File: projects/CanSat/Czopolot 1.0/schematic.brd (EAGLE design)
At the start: 35.6 x 50.8 mm, 12 parts

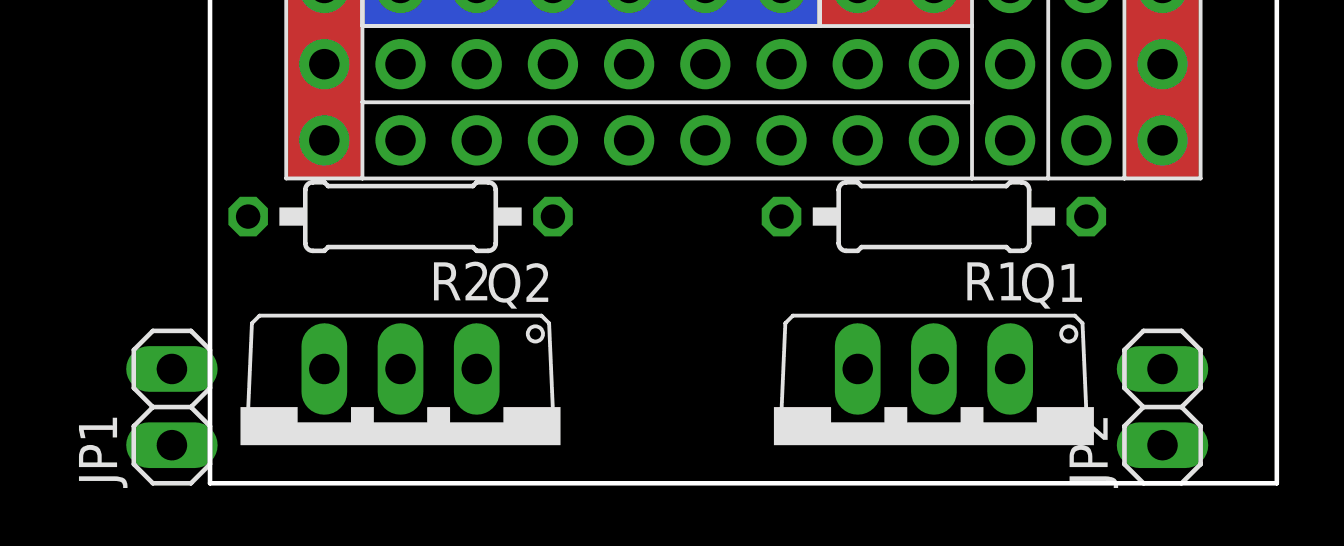
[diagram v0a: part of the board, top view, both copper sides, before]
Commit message: Work work..
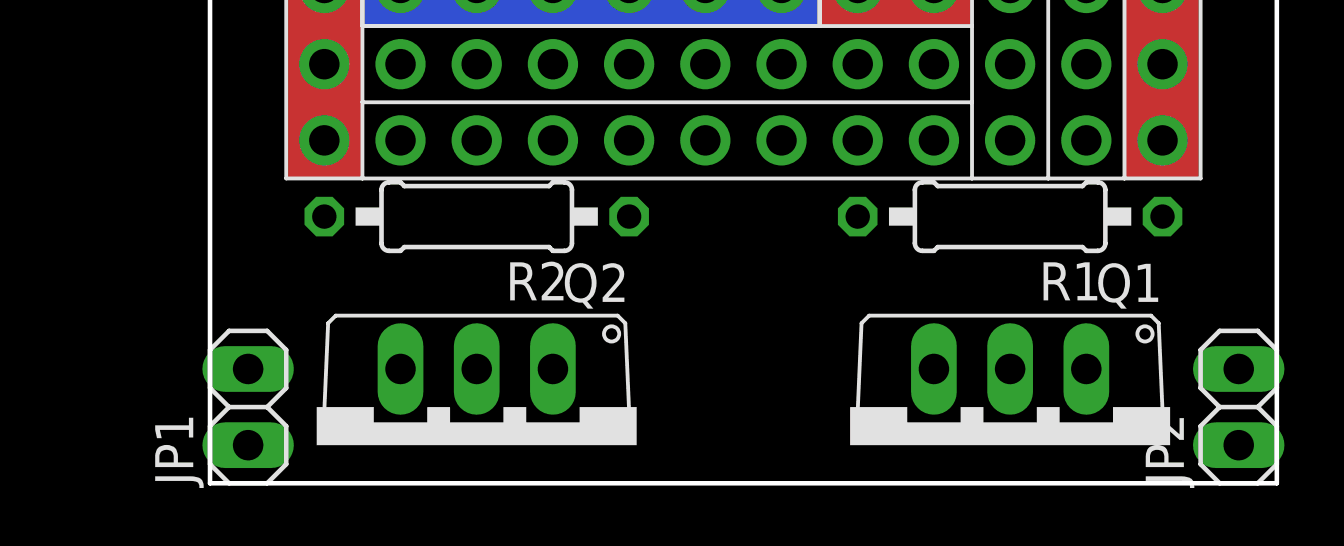
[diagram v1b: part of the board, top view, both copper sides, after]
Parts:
- moved JP1 2.54 mm to (3.81, -48.3)
- moved JP2 2.54 mm to (36.8, -48.3)
- moved Q1 2.54 mm to (29.2, -49.5)
- moved Q2 2.54 mm to (11.4, -49.5)
- moved R1 2.54 mm to (29.2, -41.9)
- moved R2 2.54 mm to (11.4, -41.9)
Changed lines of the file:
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@@
 <?xml version="1.0" encoding="utf-8"?>
 <!DOCTYPE eagle SYSTEM "eagle.dtd">
-<eagle version="9.5.2">
+<eagle version="9.5.1">
 <drawing>
 <settings>
@@
 <element name="U$3" library="SobieskiSat2" package="MODULE_MPU9250" value="MPU9250" x="20.32" y="-8.001" smashed="yes" rot="R270"/>
 <element name="U$4" library="SobieskiSat2" package="MODULE_BMP280" value="BMP280" x="15.24" y="-28.829" smashed="yes" rot="R90"/>
-<element name="R1" library="rcl" library_urn="urn:adsk.eagle:library:334" package="0207/10" package3d_urn="urn:adsk.eagle:package:23491/2" value="" x="26.67" y="-41.91" smashed="yes" rot="R180">
-<attribute name="NAME" x="29.718" y="-43.434" size="1.27" layer="25" ratio="10" rot="R180"/>
-<attribute name="POPULARITY" value="81" x="26.67" y="-41.91" size="1.778" layer="27" rot="R180" display="off"/>
-<attribute name="SPICEPREFIX" value="R" x="26.67" y="-41.91" size="1.778" layer="27" rot="R180" display="off"/>
-<attribute name="VALUE" x="28.9306" y="-41.275" size="1.27" layer="27" ratio="10" rot="R180"/>
-</element>
-<element name="R2" library="rcl" library_urn="urn:adsk.eagle:library:334" package="0207/10" package3d_urn="urn:adsk.eagle:package:23491/2" value="" x="8.89" y="-41.91" smashed="yes" rot="R180">
-<attribute name="NAME" x="11.938" y="-43.434" size="1.27" layer="25" ratio="10" rot="R180"/>
-<attribute name="POPULARITY" value="81" x="8.89" y="-41.91" size="1.778" layer="27" rot="R180" display="off"/>
-<attribute name="SPICEPREFIX" value="R" x="8.89" y="-41.91" size="1.778" layer="27" rot="R180" display="off"/>
-<attribute name="VALUE" x="11.1506" y="-41.275" size="1.27" layer="27" ratio="10" rot="R180"/>
-</element>
-<element name="Q1" library="adafruit" library_urn="urn:adsk.eagle:library:420" package="TO220V" package3d_urn="urn:adsk.eagle:package:6240882/1" value="" x="26.67" y="-49.53" smashed="yes" rot="R180">
-<attribute name="NAME" x="31.75" y="-43.4848" size="1.27" layer="25" ratio="10" rot="R180"/>
-<attribute name="VALUE" x="31.75" y="-41.91" size="1.27" layer="27" ratio="10" rot="R180"/>
-</element>
-<element name="Q2" library="adafruit" library_urn="urn:adsk.eagle:library:420" package="TO220V" package3d_urn="urn:adsk.eagle:package:6240882/1" value="" x="8.89" y="-49.53" smashed="yes" rot="R180">
-<attribute name="NAME" x="13.97" y="-43.4848" size="1.27" layer="25" ratio="10" rot="R180"/>
-<attribute name="VALUE" x="13.97" y="-41.91" size="1.27" layer="27" ratio="10" rot="R180"/>
-</element>
-<element name="JP1" library="pinhead" library_urn="urn:adsk.eagle:library:325" package="1X02" package3d_urn="urn:adsk.eagle:package:22435/2" value="" x="1.27" y="-48.26" smashed="yes" rot="R90">
-<attribute name="NAME" x="-0.5588" y="-50.8762" size="1.27" layer="25" ratio="10" rot="R90"/>
-<attribute name="POPULARITY" value="98" x="1.27" y="-48.26" size="1.778" layer="27" rot="R90" display="off"/>
-<attribute name="VALUE" x="4.445" y="-50.8" size="1.27" layer="27" rot="R90"/>
-</element>
-<element name="JP2" library="pinhead" library_urn="urn:adsk.eagle:library:325" package="1X02" package3d_urn="urn:adsk.eagle:package:22435/2" value="" x="34.29" y="-48.26" smashed="yes" rot="R90">
-<attribute name="NAME" x="32.4612" y="-50.8762" size="1.27" layer="25" ratio="10" rot="R90"/>
-<attribute name="POPULARITY" value="98" x="34.29" y="-48.26" size="1.778" layer="27" rot="R90" display="off"/>
-<attribute name="VALUE" x="37.465" y="-50.8" size="1.27" layer="27" rot="R90"/>
+<element name="R1" library="rcl" library_urn="urn:adsk.eagle:library:334" package="0207/10" package3d_urn="urn:adsk.eagle:package:23491/2" value="" x="29.21" y="-41.91" smashed="yes" rot="R180">
+<attribute name="NAME" x="32.258" y="-43.434" size="1.27" layer="25" ratio="10" rot="R180"/>
+<attribute name="POPULARITY" value="81" x="29.21" y="-41.91" size="1.778" layer="27" rot="R180" display="off"/>
+<attribute name="SPICEPREFIX" value="R" x="29.21" y="-41.91" size="1.778" layer="27" rot="R180" display="off"/>
+<attribute name="VALUE" x="31.4706" y="-41.275" size="1.27" layer="27" ratio="10" rot="R180"/>
+</element>
+<element name="R2" library="rcl" library_urn="urn:adsk.eagle:library:334" package="0207/10" package3d_urn="urn:adsk.eagle:package:23491/2" value="" x="11.43" y="-41.91" smashed="yes" rot="R180">
+<attribute name="NAME" x="14.478" y="-43.434" size="1.27" layer="25" ratio="10" rot="R180"/>
+<attribute name="POPULARITY" value="81" x="11.43" y="-41.91" size="1.778" layer="27" rot="R180" display="off"/>
+<attribute name="SPICEPREFIX" value="R" x="11.43" y="-41.91" size="1.778" layer="27" rot="R180" display="off"/>
+<attribute name="VALUE" x="13.6906" y="-41.275" size="1.27" layer="27" ratio="10" rot="R180"/>
+</element>
+<element name="Q1" library="adafruit" library_urn="urn:adsk.eagle:library:420" package="TO220V" package3d_urn="urn:adsk.eagle:package:6240882/1" value="" x="29.21" y="-49.53" smashed="yes" rot="R180">
+<attribute name="NAME" x="34.29" y="-43.4848" size="1.27" layer="25" ratio="10" rot="R180"/>
+<attribute name="VALUE" x="34.29" y="-41.91" size="1.27" layer="27" ratio="10" rot="R180"/>
+</element>
+<element name="Q2" library="adafruit" library_urn="urn:adsk.eagle:library:420" package="TO220V" package3d_urn="urn:adsk.eagle:package:6240882/1" value="" x="11.43" y="-49.53" smashed="yes" rot="R180">
+<attribute name="NAME" x="16.51" y="-43.4848" size="1.27" layer="25" ratio="10" rot="R180"/>
+<attribute name="VALUE" x="16.51" y="-41.91" size="1.27" layer="27" ratio="10" rot="R180"/>
+</element>
+<element name="JP1" library="pinhead" library_urn="urn:adsk.eagle:library:325" package="1X02" package3d_urn="urn:adsk.eagle:package:22435/2" value="" x="3.81" y="-48.26" smashed="yes" rot="R90">
+<attribute name="NAME" x="1.9812" y="-50.8762" size="1.27" layer="25" ratio="10" rot="R90"/>
+<attribute name="POPULARITY" value="98" x="3.81" y="-48.26" size="1.778" layer="27" rot="R90" display="off"/>
+<attribute name="VALUE" x="6.985" y="-50.8" size="1.27" layer="27" rot="R90"/>
+</element>
+<element name="JP2" library="pinhead" library_urn="urn:adsk.eagle:library:325" package="1X02" package3d_urn="urn:adsk.eagle:package:22435/2" value="" x="36.83" y="-48.26" smashed="yes" rot="R90">
+<attribute name="NAME" x="35.0012" y="-50.8762" size="1.27" layer="25" ratio="10" rot="R90"/>
+<attribute name="POPULARITY" value="98" x="36.83" y="-48.26" size="1.778" layer="27" rot="R90" display="off"/>
+<attribute name="VALUE" x="40.005" y="-50.8" size="1.27" layer="27" rot="R90"/>
 </element>
 </elements>
@@
 <wire x1="3.81" y1="-3.81" x2="6.35" y2="-3.81" width="0" layer="19" extent="1-1"/>
 </signal>
-<signal name="GND">
+<signal name="GND" airwireshidden="yes">
 <contactref element="ULTIMATE_GPS" pad="2"/>
 <contactref element="U$2" pad="GND@1"/>
@@
 <wire x1="11.43" y1="-19.05" x2="17.13" y2="-23.51" width="0" layer="19" extent="1-1"/>
 </signal>
-<signal name="VCC">
+<signal name="VCC" airwireshidden="yes">
 <contactref element="U$2" pad="VCC"/>
 <contactref element="U$3" pad="VCC"/>
@@
 <wire x1="34.29" y1="-34.29" x2="31.13" y2="-23.51" width="0" layer="19" extent="1-1"/>
 </signal>
-<signal name="V+">
+<signal name="V+" airwireshidden="yes">
 <contactref element="U$1" pad="V+3"/>
 <contactref element="U$1" pad="V+2"/>
